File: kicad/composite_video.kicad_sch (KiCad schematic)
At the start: 1 part, among them J10 Composite Jack

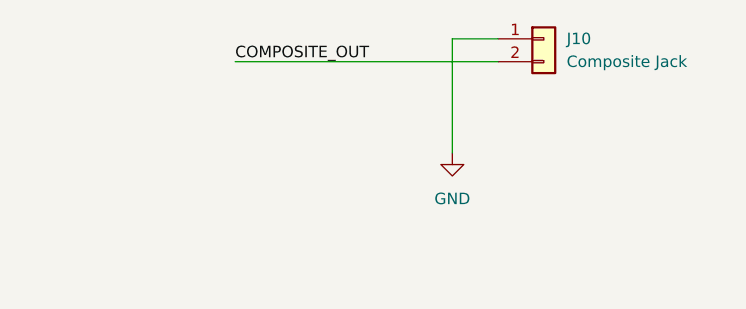
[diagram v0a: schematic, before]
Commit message: update kicad project
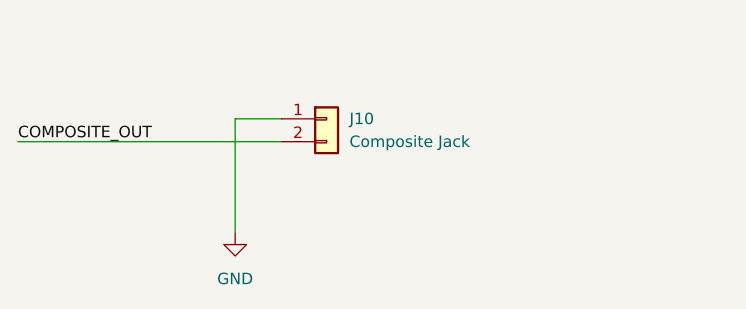
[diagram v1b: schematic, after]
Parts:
- J10: seq_coord (none) -> J33
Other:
- moved on the sheet: J10
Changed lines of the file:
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@@
 	(wire
 		(pts
-			(xy 140.97 78.74) (xy 170.18 78.74)
+			(xy 116.84 87.63) (xy 146.05 87.63)
 		)
 		(stroke
@@
 	(wire
 		(pts
-			(xy 165.1 76.2) (xy 165.1 88.9)
+			(xy 140.97 85.09) (xy 140.97 97.79)
 		)
 		(stroke
@@
 	(wire
 		(pts
-			(xy 165.1 76.2) (xy 170.18 76.2)
+			(xy 140.97 85.09) (xy 146.05 85.09)
 		)
 		(stroke
@@
 	)
 	(label "COMPOSITE_OUT"
-		(at 140.97 78.74 0)
+		(at 116.84 87.63 0)
 		(effects
 			(font
@@
 	(symbol
 		(lib_id "Connector_Generic:Conn_01x02")
-		(at 175.26 76.2 0)
+		(at 151.13 85.09 0)
 		(unit 1)
 		(exclude_from_sim no)
@@
 		(dnp no)
 		(property "Reference" "J10"
-			(at 177.8 76.1999 0)
+			(at 153.67 85.0899 0)
 			(effects
 				(font
@@
 		)
 		(property "Value" "Composite Jack"
-			(at 177.8 78.7399 0)
+			(at 153.67 87.6299 0)
 			(effects
 				(font
@@
 		)
 		(property "Footprint" "Connector_PinHeader_2.54mm:PinHeader_1x02_P2.54mm_Horizontal"
-			(at 175.26 76.2 0)
+			(at 151.13 85.09 0)
 			(effects
 				(font
@@
 		)
 		(property "Datasheet" "~"
-			(at 175.26 76.2 0)
+			(at 151.13 85.09 0)
 			(effects
 				(font
@@
 		)
 		(property "Description" "Generic connector, single row, 01x02, script generated (kicad-library-utils/schlib/autogen/connector/)"
-			(at 175.26 76.2 0)
+			(at 151.13 85.09 0)
 			(effects
 				(font
@@
 		)
 		(property "seq_partno" ""
-			(at 175.26 76.2 0)
+			(at 151.13 85.09 0)
 			(effects
 				(font
@@
 			)
 		)
-		(property "seq_coord" ""
-			(at 175.26 76.2 0)
+		(property "seq_coord" "J33"
+			(at 151.13 85.09 0)
 			(effects
 				(font
@@
 		)
 		(property "seq_silkscreen" ""
-			(at 175.26 76.2 0)
+			(at 151.13 85.09 0)
 			(effects
 				(font
@@
 		)
 		(property "seq_sharpie" ""
-			(at 175.26 76.2 0)
+			(at 151.13 85.09 0)
 			(effects
 				(font
@@
 		)
 		(property "seq_notes" ""
-			(at 175.26 76.2 0)
+			(at 151.13 85.09 0)
 			(effects
 				(font
@@
 	(symbol
 		(lib_id "power:GND")
-		(at 165.1 88.9 0)
+		(at 140.97 97.79 0)
 		(unit 1)
 		(exclude_from_sim no)
@@
 		(fields_autoplaced yes)
 		(property "Reference" "#PWR075"
-			(at 165.1 95.25 0)
+			(at 140.97 104.14 0)
 			(effects
 				(font
@@
 		)
 		(property "Value" "GND"
-			(at 165.1 93.98 0)
+			(at 140.97 102.87 0)
 			(effects
 				(font
@@
 		)
 		(property "Footprint" ""
-			(at 165.1 88.9 0)
+			(at 140.97 97.79 0)
 			(effects
 				(font
@@
 		)
 		(property "Datasheet" ""
-			(at 165.1 88.9 0)
+			(at 140.97 97.79 0)
 			(effects
 				(font
@@
 		)
 		(property "Description" "Power symbol creates a global label with name \"GND\" , ground"
-			(at 165.1 88.9 0)
+			(at 140.97 97.79 0)
 			(effects
 				(font
